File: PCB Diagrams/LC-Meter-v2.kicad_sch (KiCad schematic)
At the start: 32 parts, among them J1 Power, J2 External, J3 Cx/Lx, J4 GND, J5 Display I2C, J6 Base 01, J7 Top 01, J8 Base 02, J9 Top 02, SW1 Select, SW2 High, SW3 Med, SW4 Low, U1 LM358

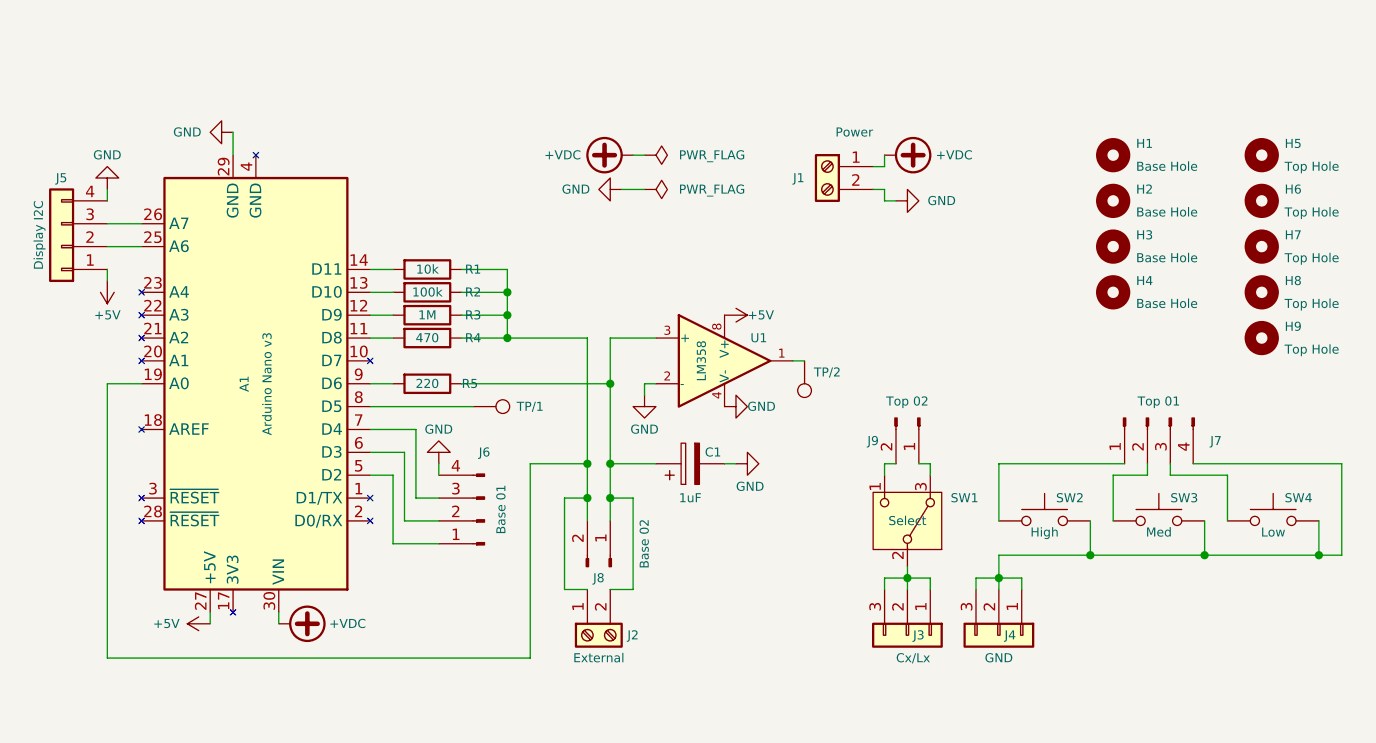
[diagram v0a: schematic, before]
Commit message: first commit
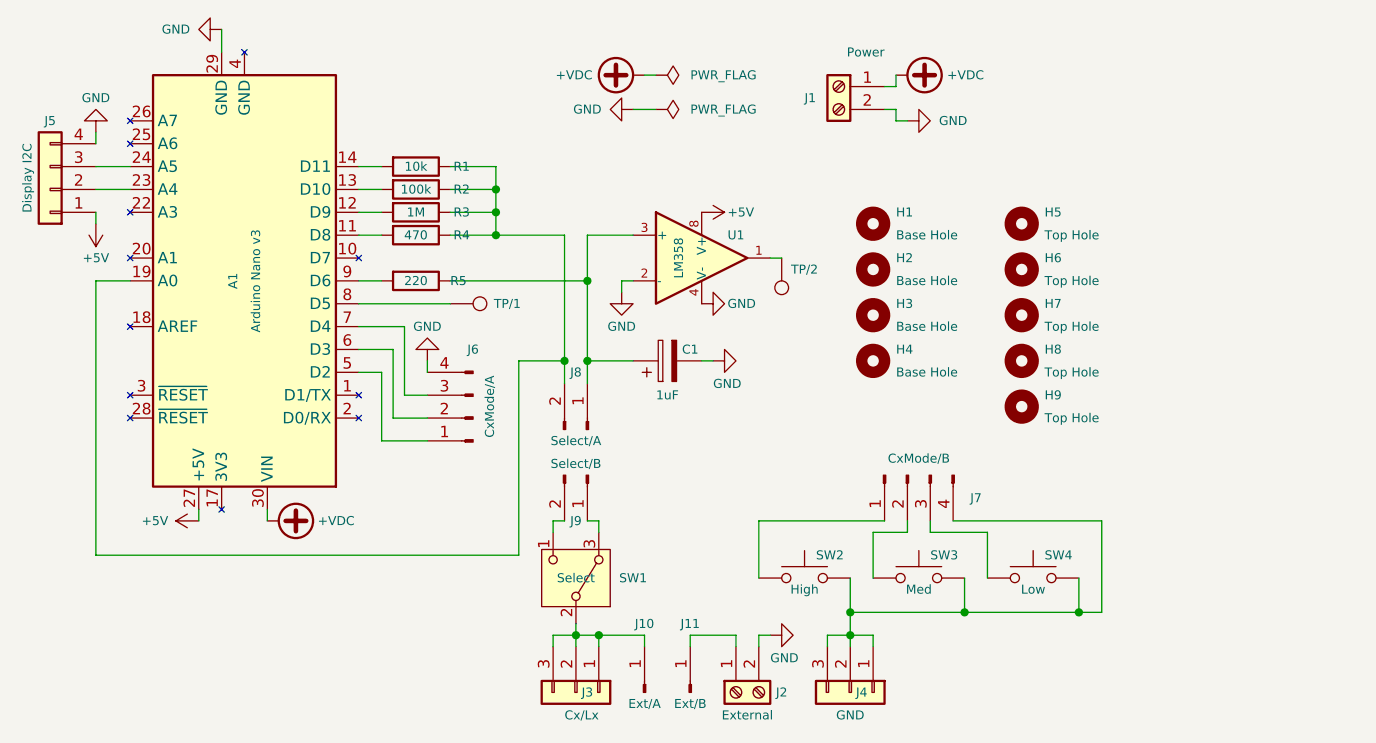
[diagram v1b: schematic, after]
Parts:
- added J10: Ext/A, Connector_PinHeader_2.54mm:PinHeader_1x01_P2.54mm_Horizontal, symbol Connector:Conn_01x01_Pin
- added J11: Ext/B, Connector_PinHeader_2.54mm:PinHeader_1x01_P2.54mm_Horizontal, symbol Connector:Conn_01x01_Pin
- J6: value Base 01 -> CxMode/A
- J7: value Top 01 -> CxMode/B
- J8: value Base 02 -> Select/A
- J9: value Top 02 -> Select/B
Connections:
- net GND: now also J2.2 (Pin_2)
- net at J5.2 (Pin_2): now also A1.23 (A4); no longer A1.25 (A6)
- net at J5.3 (Pin_3): now also A1.24 (A5); no longer A1.26 (A7)
- net at C1.1, J8.1 (Pin_1), R5.1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: no longer J2.2 (Pin_2)
- net at J3.1 (Pin_1), J3.2 (Pin_2), J3.3 (Pin_3)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: now also J10.1 (Pin_1)
- net at A1.19 (A0), J8.2 (Pin_2), R1.1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: no longer J2.1 (Pin_1)
- new net: J11.1 (Pin_1), J2.1 (Pin_1)
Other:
- moved on the sheet: A1, C1, H1, H2, H3, H4, H5, H6, H7, H8, H9, J1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
